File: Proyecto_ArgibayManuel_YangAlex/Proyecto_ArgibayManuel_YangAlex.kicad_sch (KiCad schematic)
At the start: 38 parts, among them IC1 LM1117, J2 Conn_01x04, J3 Conn_01x06, J4 Conn_01x04, SW1 SW_Push, SW2 SW_Push, SW3 SW_Push, SW4 SW_Push, U1 PIC18F258-I_SO, U10 LT1716IS5TRMPBF, U6 MCP2551-I-P, U9 LT1716IS5TRMPBF, X1 DB9, X2 DB9, Y1 Crystal

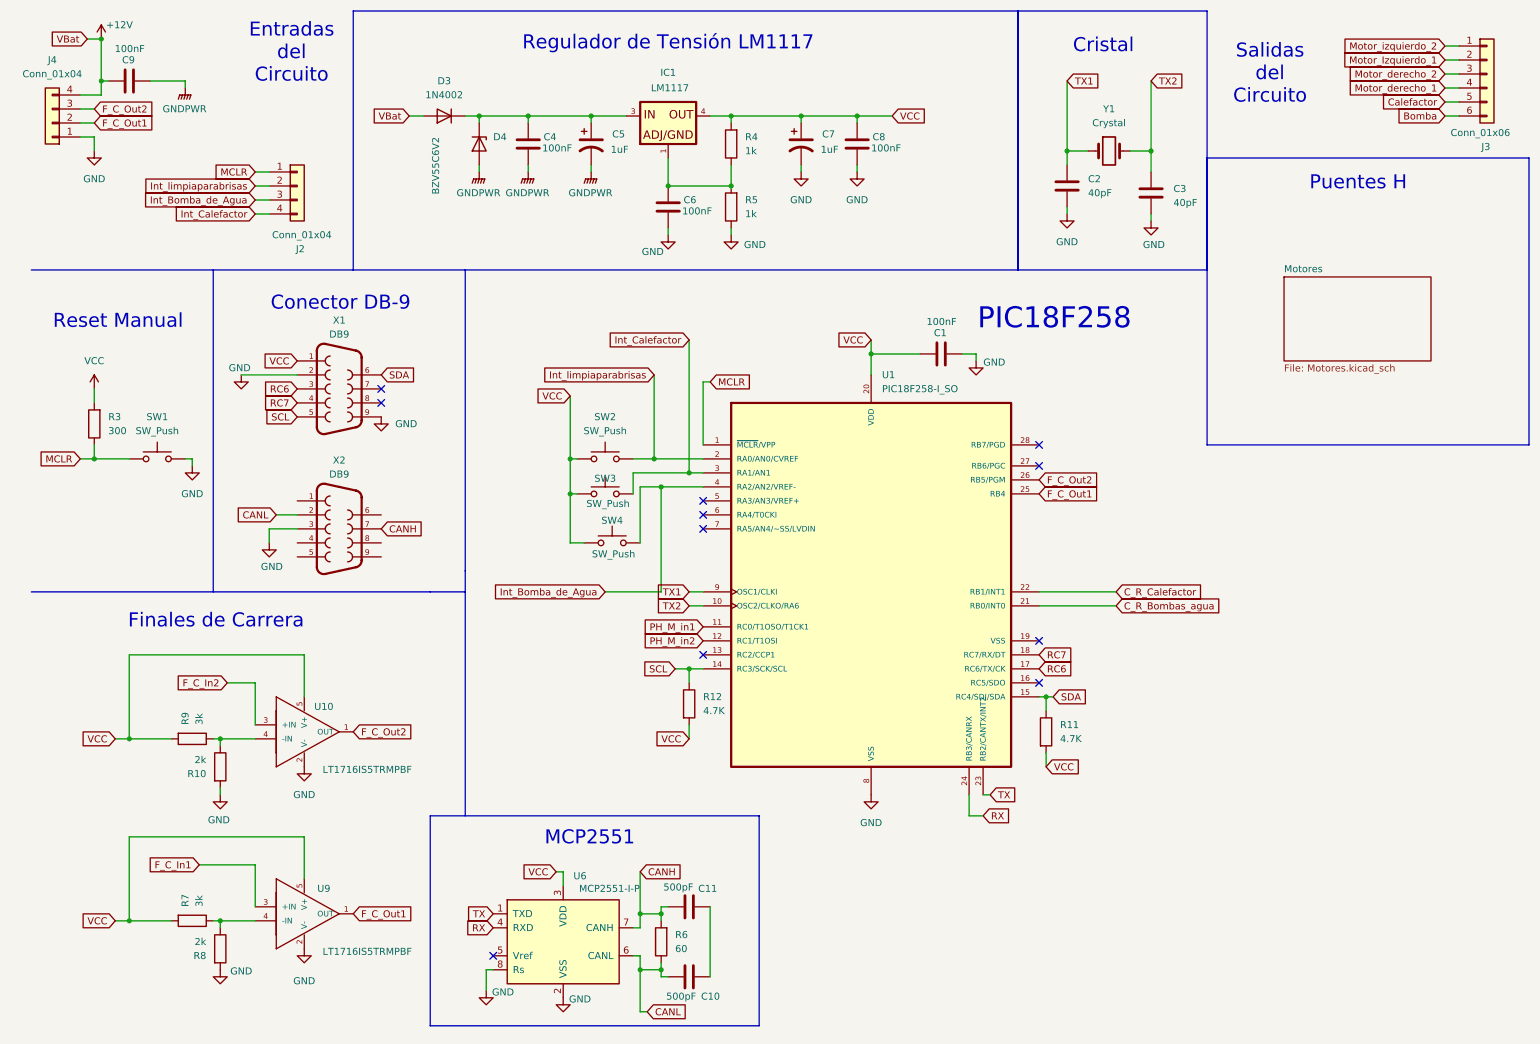
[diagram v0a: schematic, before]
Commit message: Ordenar esquematico
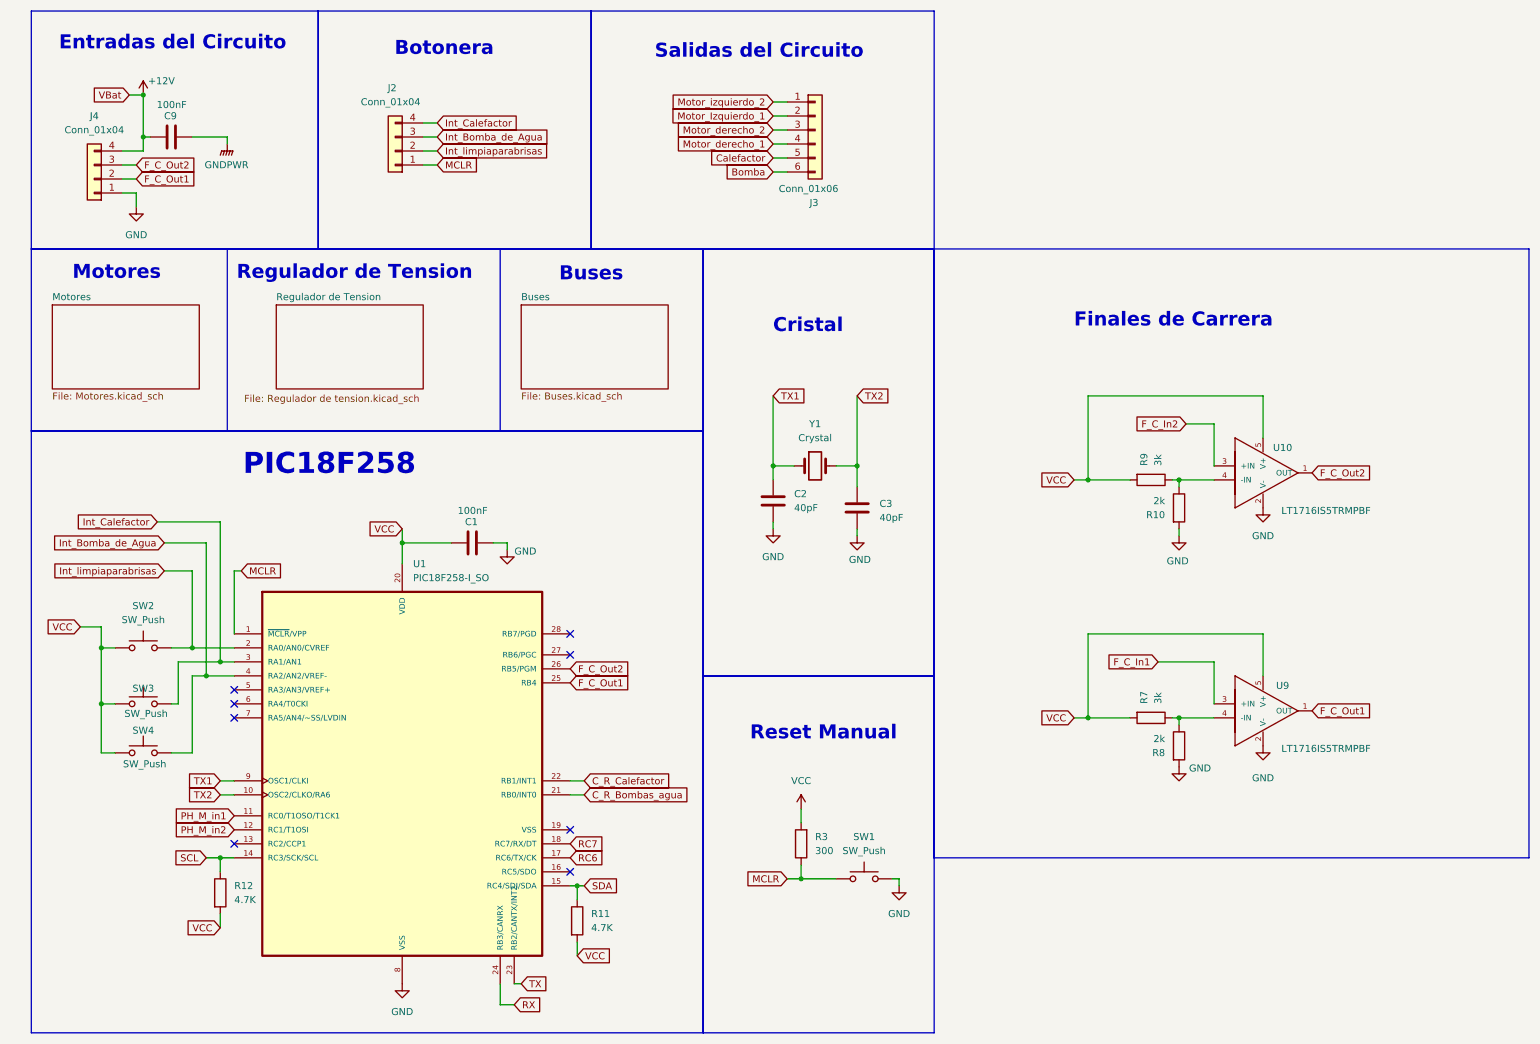
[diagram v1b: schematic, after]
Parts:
- removed C10, C11: 500pF, symbol Device:C
- removed C4, C6, C8: 100nF, symbol Device:C
- removed C5, C7: 1uF, symbol Device:C_Polarized_US
- removed D3: 1N4002, Diode_THT:D_DO-41_SOD81_P10.16mm_Horizontal, symbol Diode:1N4002
- removed D4: BZV55C6V2, Diode_SMD:D_MiniMELF, symbol Diode:BZV55C6V2
- removed IC1: LM1117, symbol LM1117:LM1117
- removed R4, R5: 1k, symbol Device:R
- removed R6: 60, symbol Device:R
- removed U6: MCP2551-I-P, Package_DIP:DIP-8_W7.62mm, symbol Interface_CAN_LIN:MCP2551-I-P
- removed X1, X2: DB9, DB9:DB9, symbol DB9:DB9
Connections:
- no-connect marks 11 -> 8
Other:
- added sheet Buses (Buses.kicad_sch)
- added sheet Regulador de Tension (Regulador de tension.kicad_sch)
- note added: "Botonera"
- note added: "Buses"
- note added: "Motores"
- note added: "Regulador de Tension"
- note removed: "Conector DB-9"
- note removed: "MCP2551"
- note removed: "Puentes H"
- note removed: "Regulador de Tensión LM1117"
- moved on the sheet: C1, C2, C3, C9, J2, J3, J4, R10, R11, R12, R3, R7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
